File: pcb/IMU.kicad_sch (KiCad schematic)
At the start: 8 parts, among them U1 ICM-42688-P

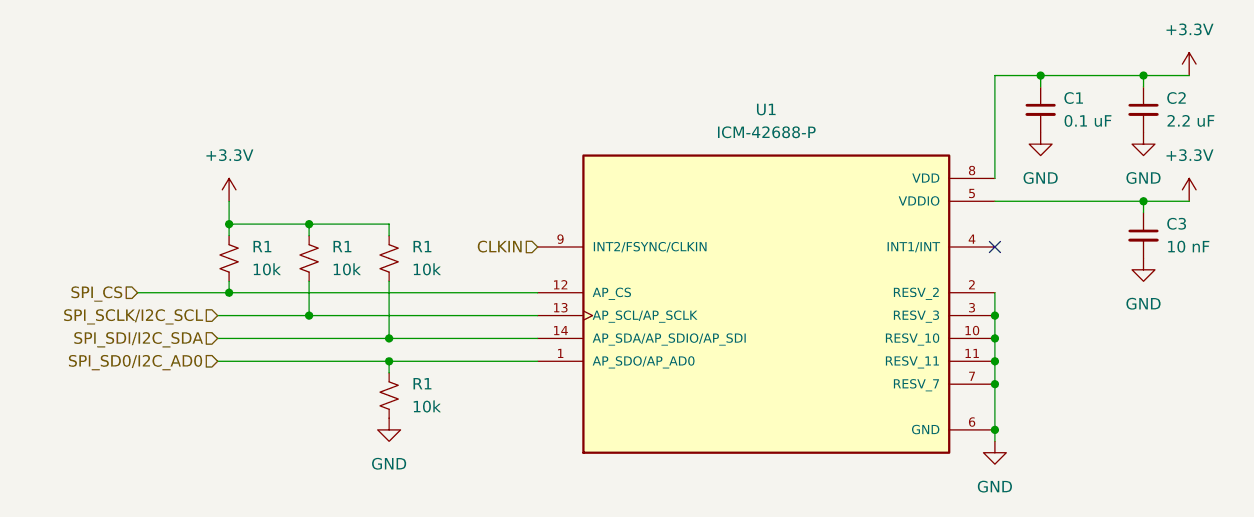
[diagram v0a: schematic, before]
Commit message: Add files via upload
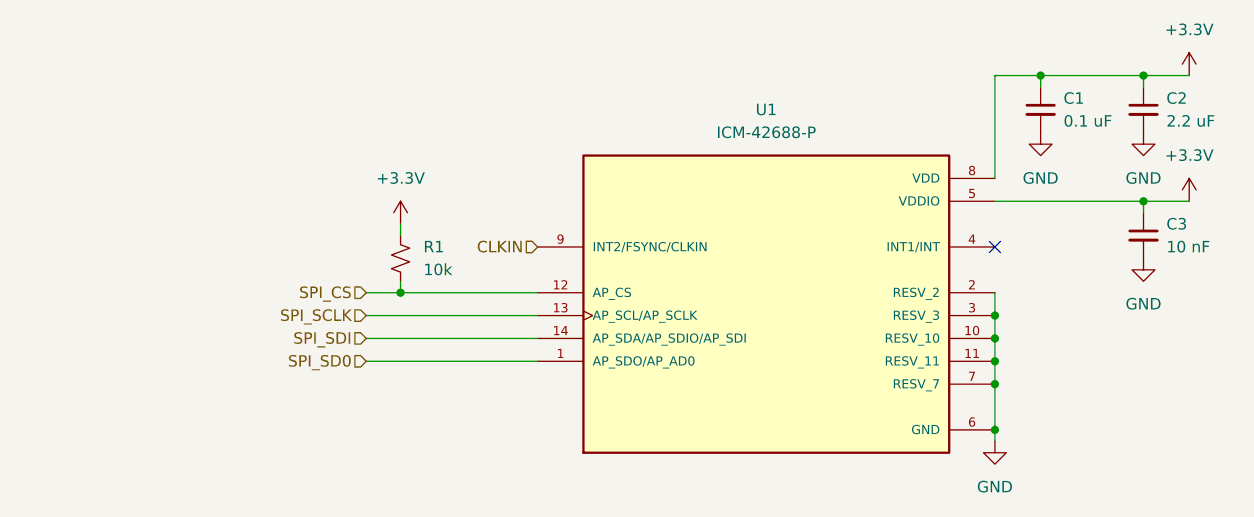
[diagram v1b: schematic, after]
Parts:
- removed R1 (x3): 10k, Resistor_SMD:R_0805_2012Metric, symbol Device:R_Small_US
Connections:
- net SPI_SCLK/I2C_SCL renamed SPI_SCLK
- net SPI_SD0/I2C_AD0 renamed SPI_SD0
- net SPI_SDI/I2C_SDA renamed SPI_SDI
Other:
- moved on the sheet: R1
